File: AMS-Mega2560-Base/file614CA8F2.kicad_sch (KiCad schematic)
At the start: 22 parts, among them IC13 MAX764CPA+, IC14 LM2917N-8_NOPB, J23 Conn_01x02, J24 Conn_01x02, J31 Conn_01x02, K1 DIP05-1A72-12L, Q25 2N7000

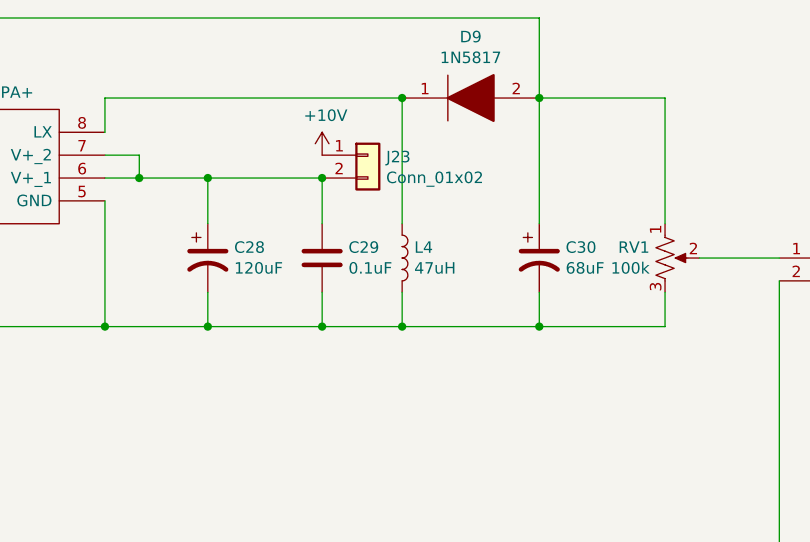
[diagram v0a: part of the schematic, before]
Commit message: not sure what i changed i'm pushing these up since this branch may be deleted
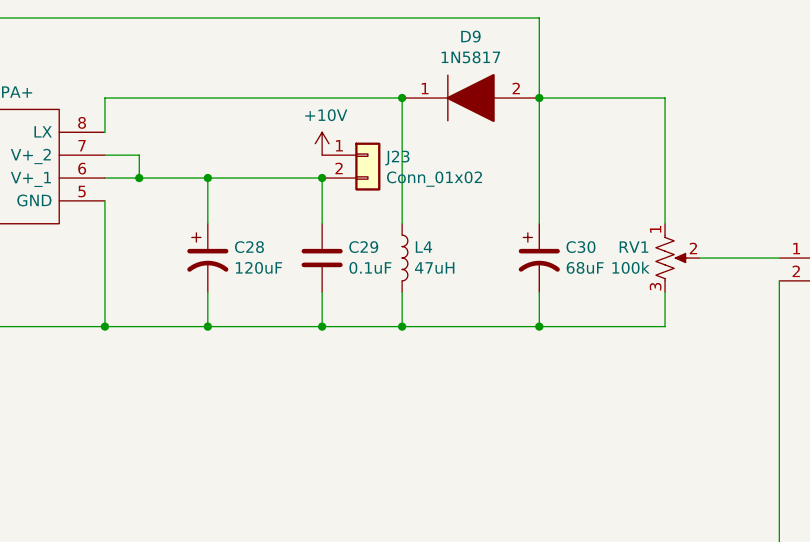
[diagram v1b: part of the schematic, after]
